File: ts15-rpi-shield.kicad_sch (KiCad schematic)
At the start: 13 parts, among them CON1 TROPIC01, IC1 TROPIC01_chip, J1 RPI socket

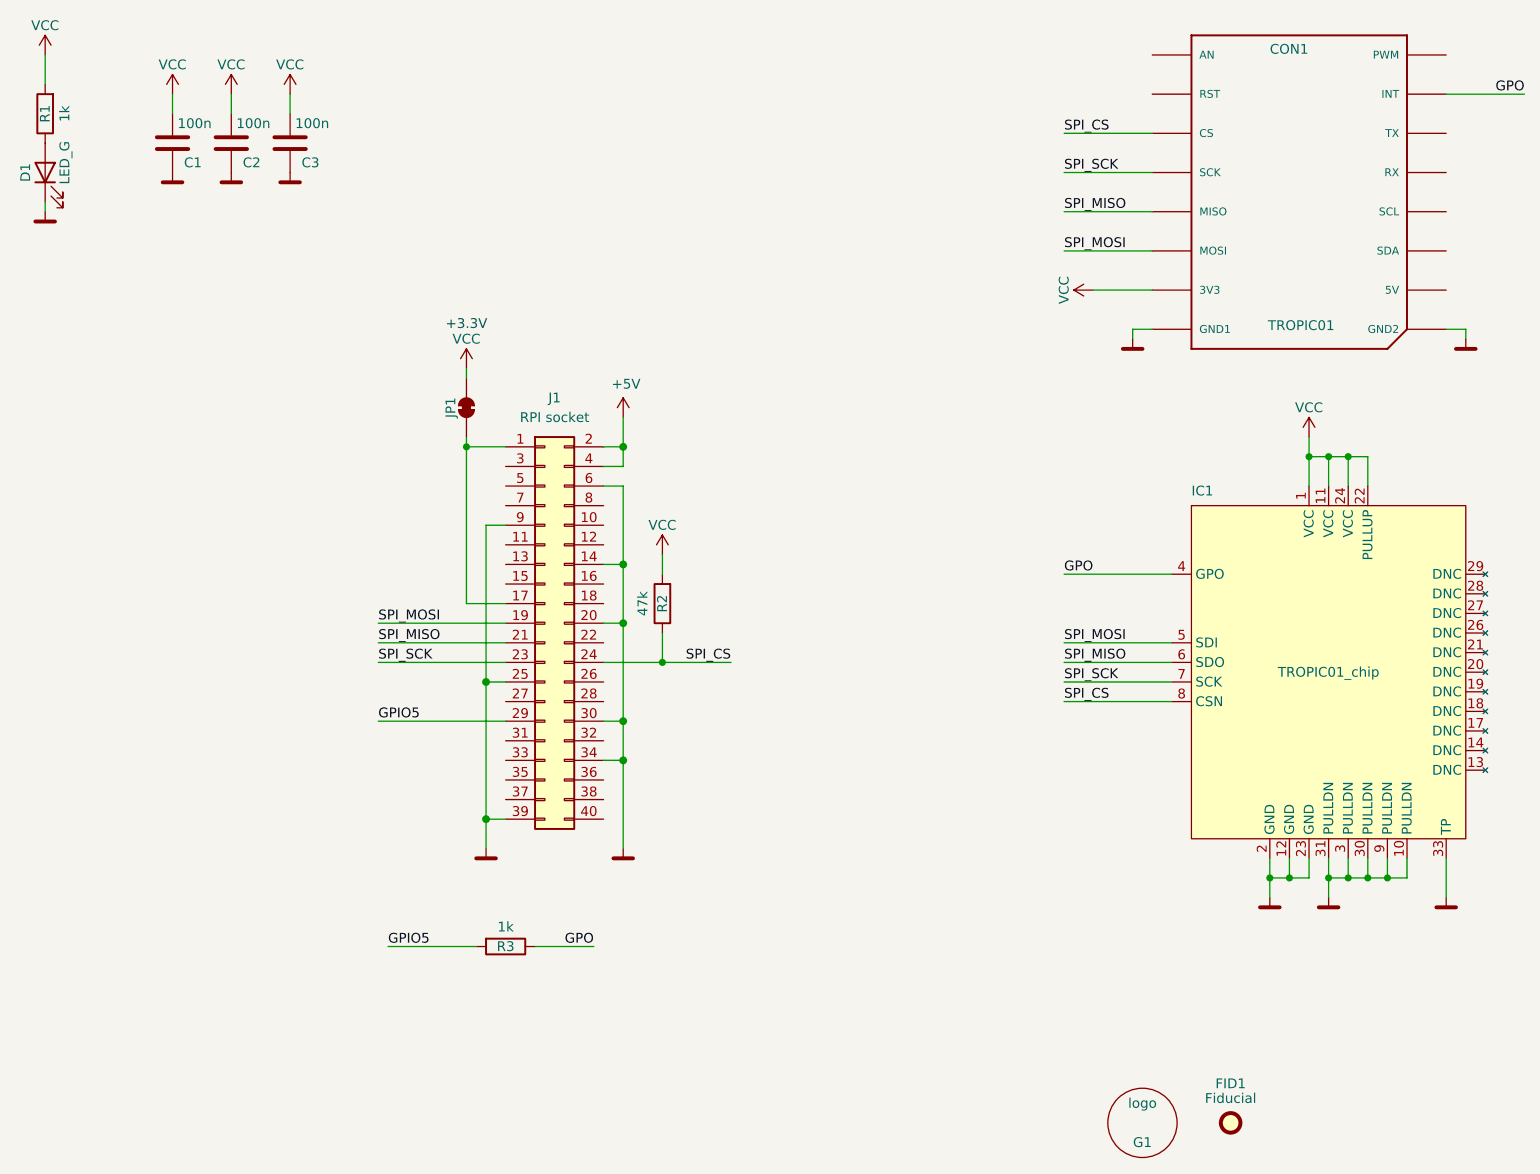
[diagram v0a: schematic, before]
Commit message: project: Add fabrication gerber data and some tuning
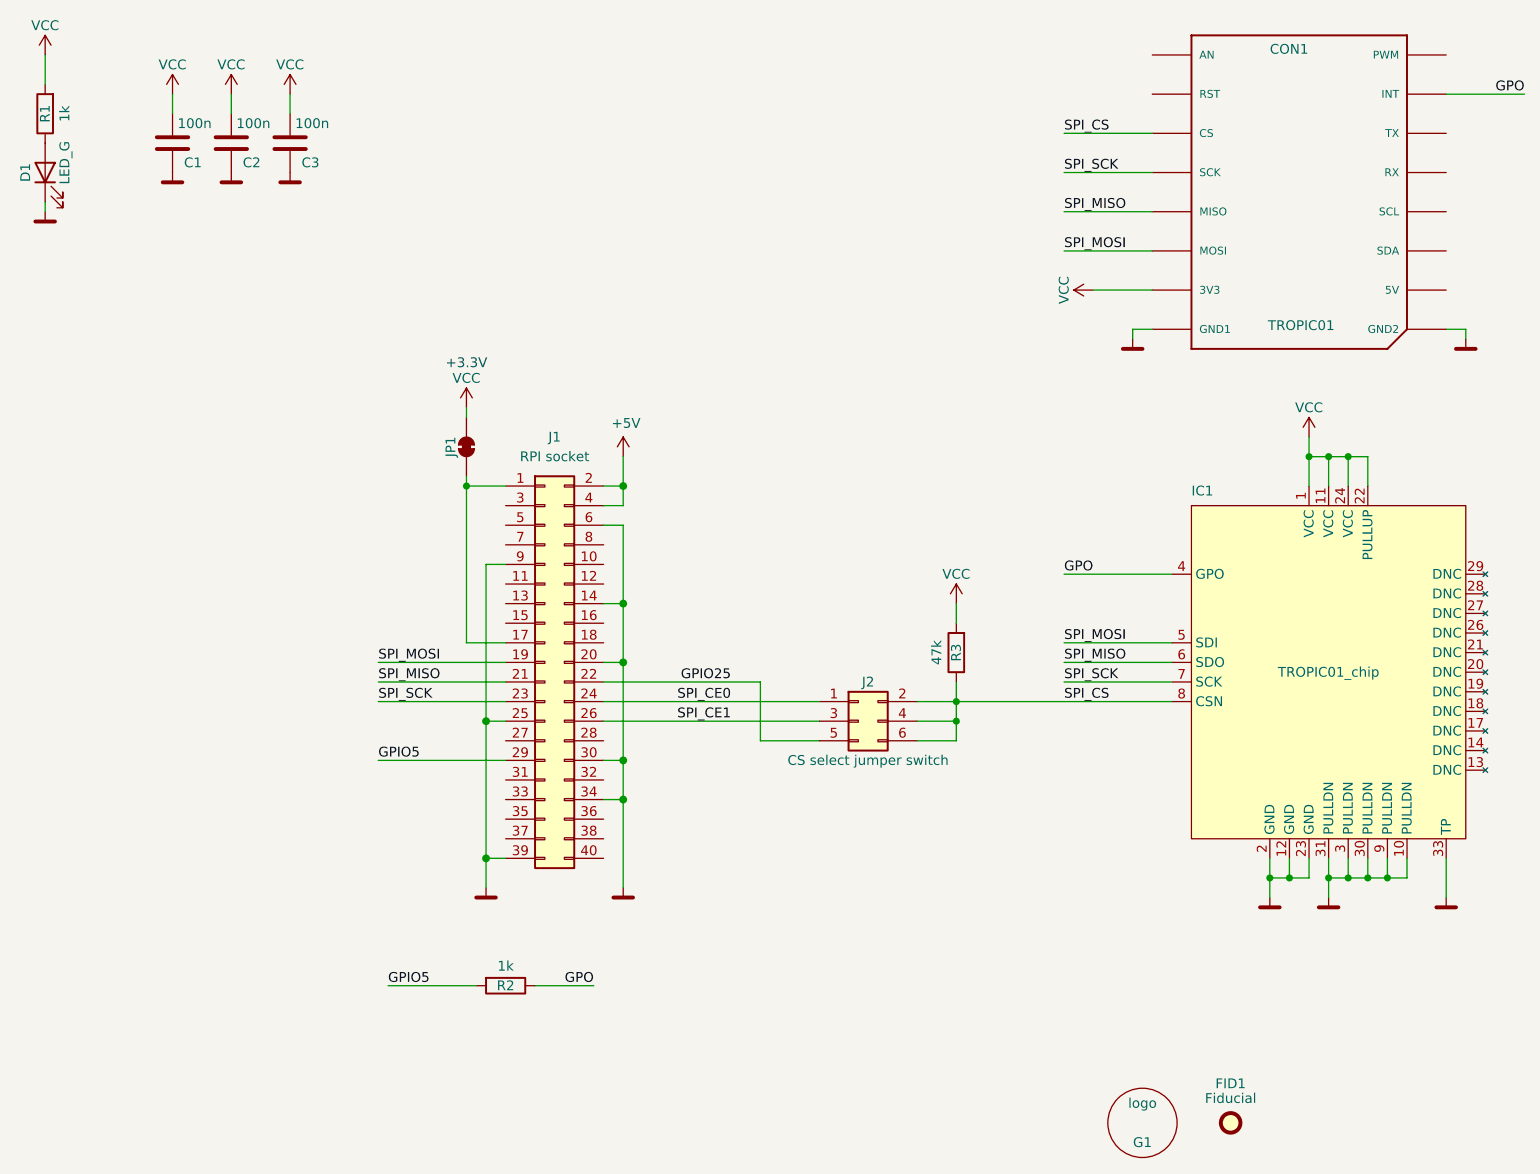
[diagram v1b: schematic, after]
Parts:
- added J2: CS select jumper switch, Connector_PinHeader_2.54mm:PinHeader_2x03_P2.54mm_Vertical, symbol Connector_Generic:Conn_02x03_Odd_Even
- renumbered R3 to R2, R2 to R3
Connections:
- net SPI_CS: now also J2.2 (Pin_2), J2.4 (Pin_4), J2.6 (Pin_6); no longer J1.24 (Pin_24)
- net GPIO25: now reaches J1.22 (Pin_22)
- net GPIO25: now also J2.5 (Pin_5)
- net SPI_CE1: now reaches J1.26 (Pin_26)
- net SPI_CE1: now also J2.3 (Pin_3)
- new net SPI_CE0: J1.24 (Pin_24), J2.1 (Pin_1)
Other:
- moved on the sheet: J1, JP1, R2, R3
